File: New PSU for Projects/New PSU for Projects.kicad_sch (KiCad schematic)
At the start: 43 parts, among them IC4 LF351DT, J1 Toroid 5VA/15V, J2 240V Mains, J3 Current Flow Test Point, J4 PVG3A202C01R00, Q1 BC848, Q2 BC848, U3 SN74HC74N

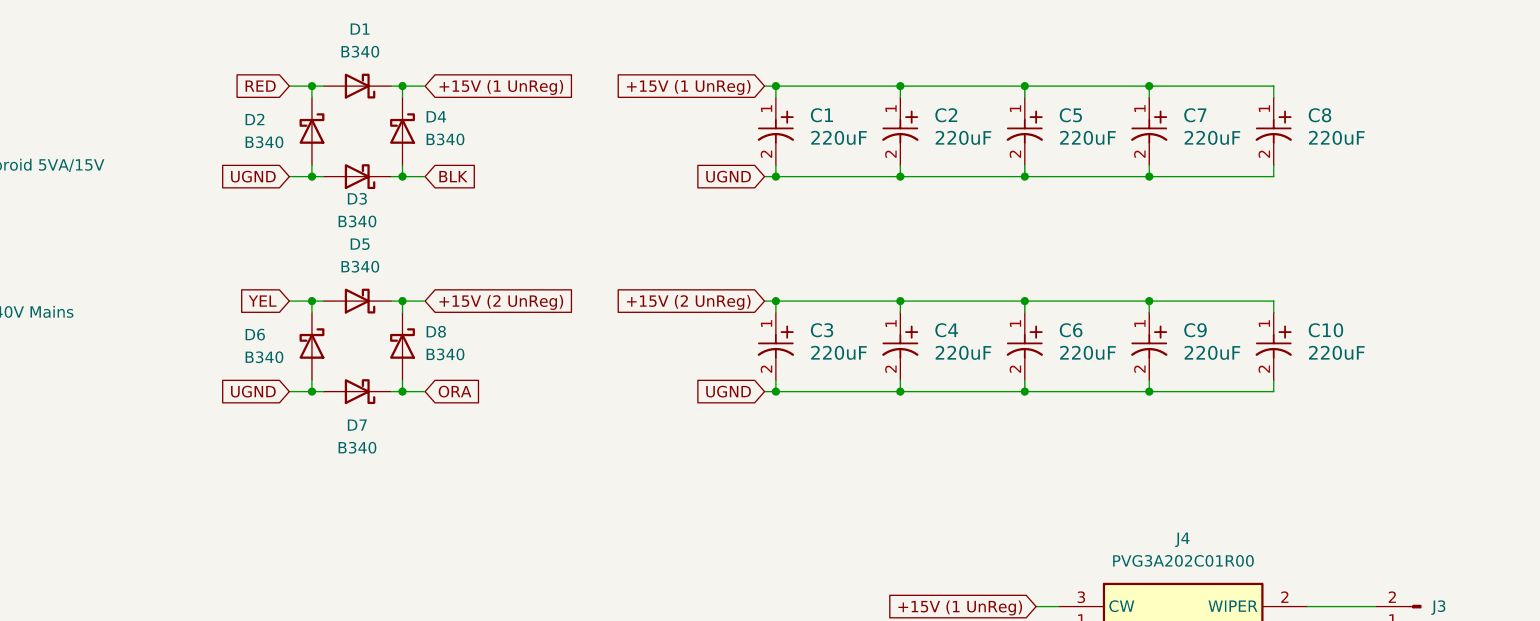
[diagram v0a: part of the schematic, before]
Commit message: A few minor changes
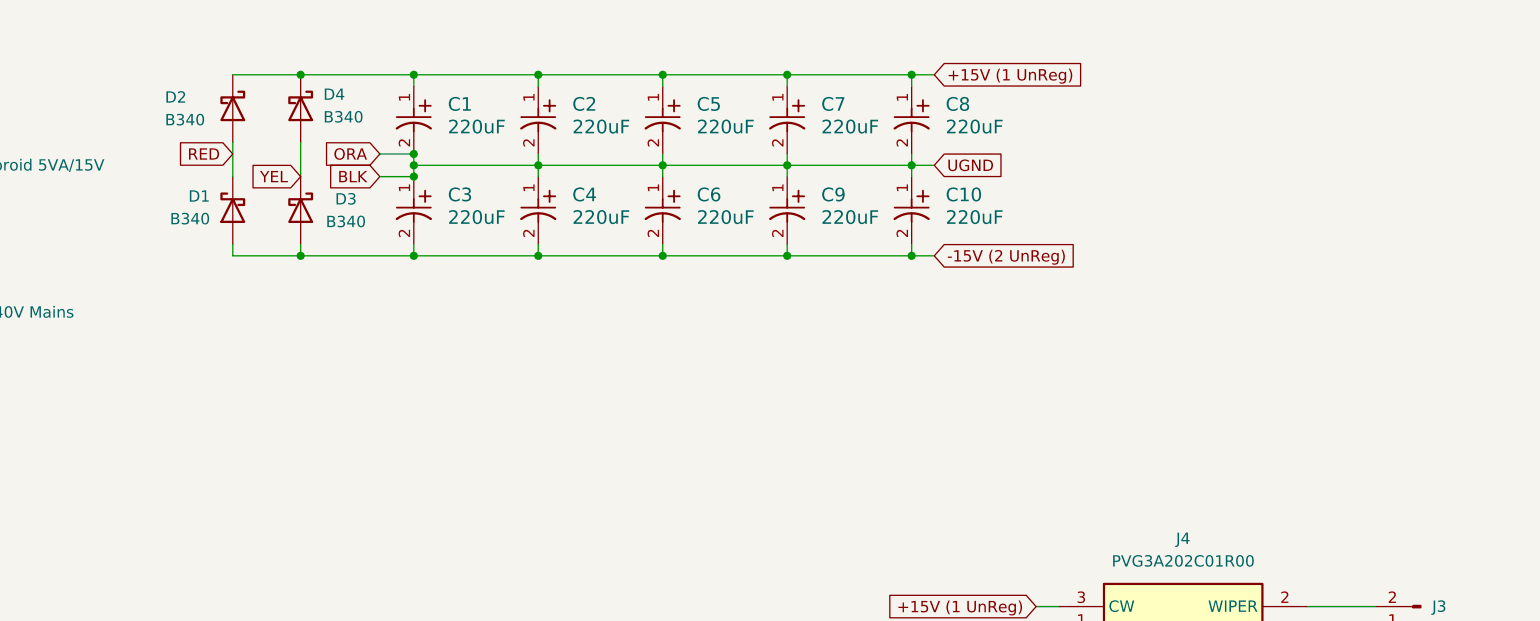
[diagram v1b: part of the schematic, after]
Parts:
- removed D5, D6, D7, D8: B340, Diode_SMD:D_SMC, symbol Diode:B340
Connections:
- net +15V (2 UnReg) is gone; now on net BLK: C10.1, C3.1, C4.1, C6.1, C9.1
- net ORA is gone; now on net BLK: J1.4 (Pin_4)
- net +15V (1 UnReg): now also D2.1 (K); no longer D1.1 (K)
- net BLK: now also C1.2, C13.2, C14.2, C2.2, C3.1, C5.1, C5.2, C7.2, C8.2, IC4.4 (VCC-), Q1.2 (E), Q2.2 (E), R2.1, U3.7 (GND), Z9.2 (A); no longer D3.1 (K), D4.2 (A)
- net RED: now also D1.1 (K), D2.2 (A); no longer D1.2 (A), D2.1 (K)
- net YEL: now also D3.1 (K), D4.2 (A)
- removed net UGND: C1.2, C10.2, C13.2, C14.2, C2.2, C3.1, C3.2, C4.2, C5.1, C5.2, C6.2, C7.2, C8.2, C9.2, D2.2 (A), D3.2 (A), IC4.4 (VCC-), Q1.2 (E), Q2.2 (E), R2.1, U3.7 (GND), Z9.2 (A)
- new net -15V (2 UnReg): C10.2, C3.2, C4.2, C6.2, C9.2, D1.2 (A), D3.2 (A)
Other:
- moved on the sheet: C1, C10, C2, C3, C4, C5, C6, C7, C8, C9, D1, D2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

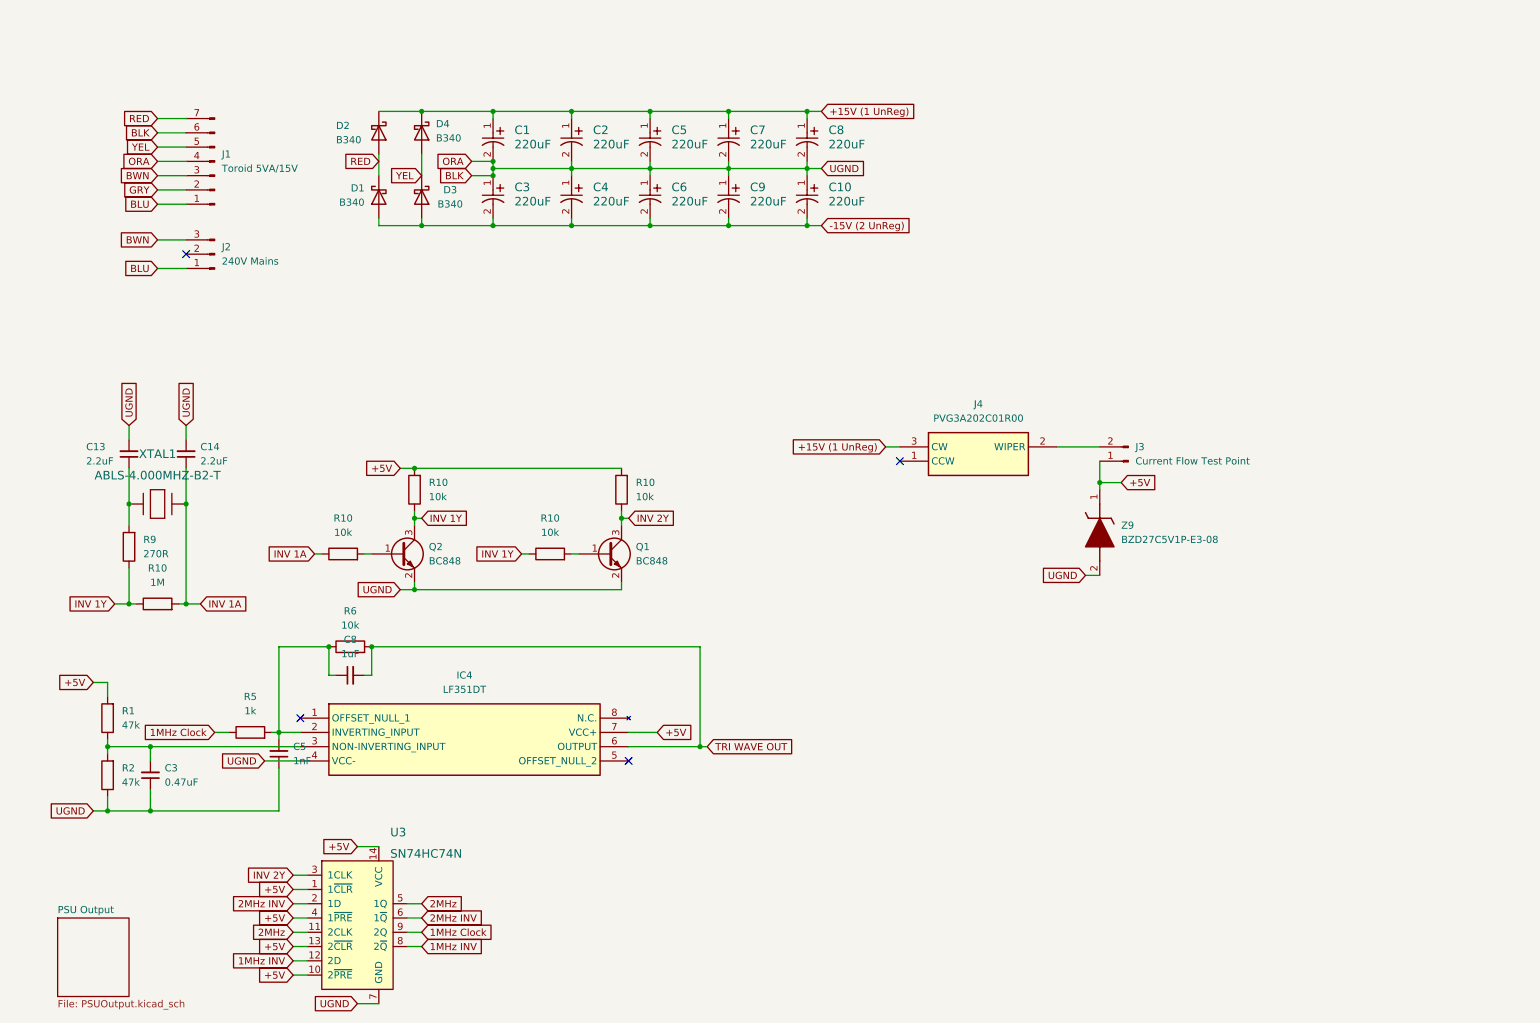
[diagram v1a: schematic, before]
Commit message: Lyrebird Initial Upload
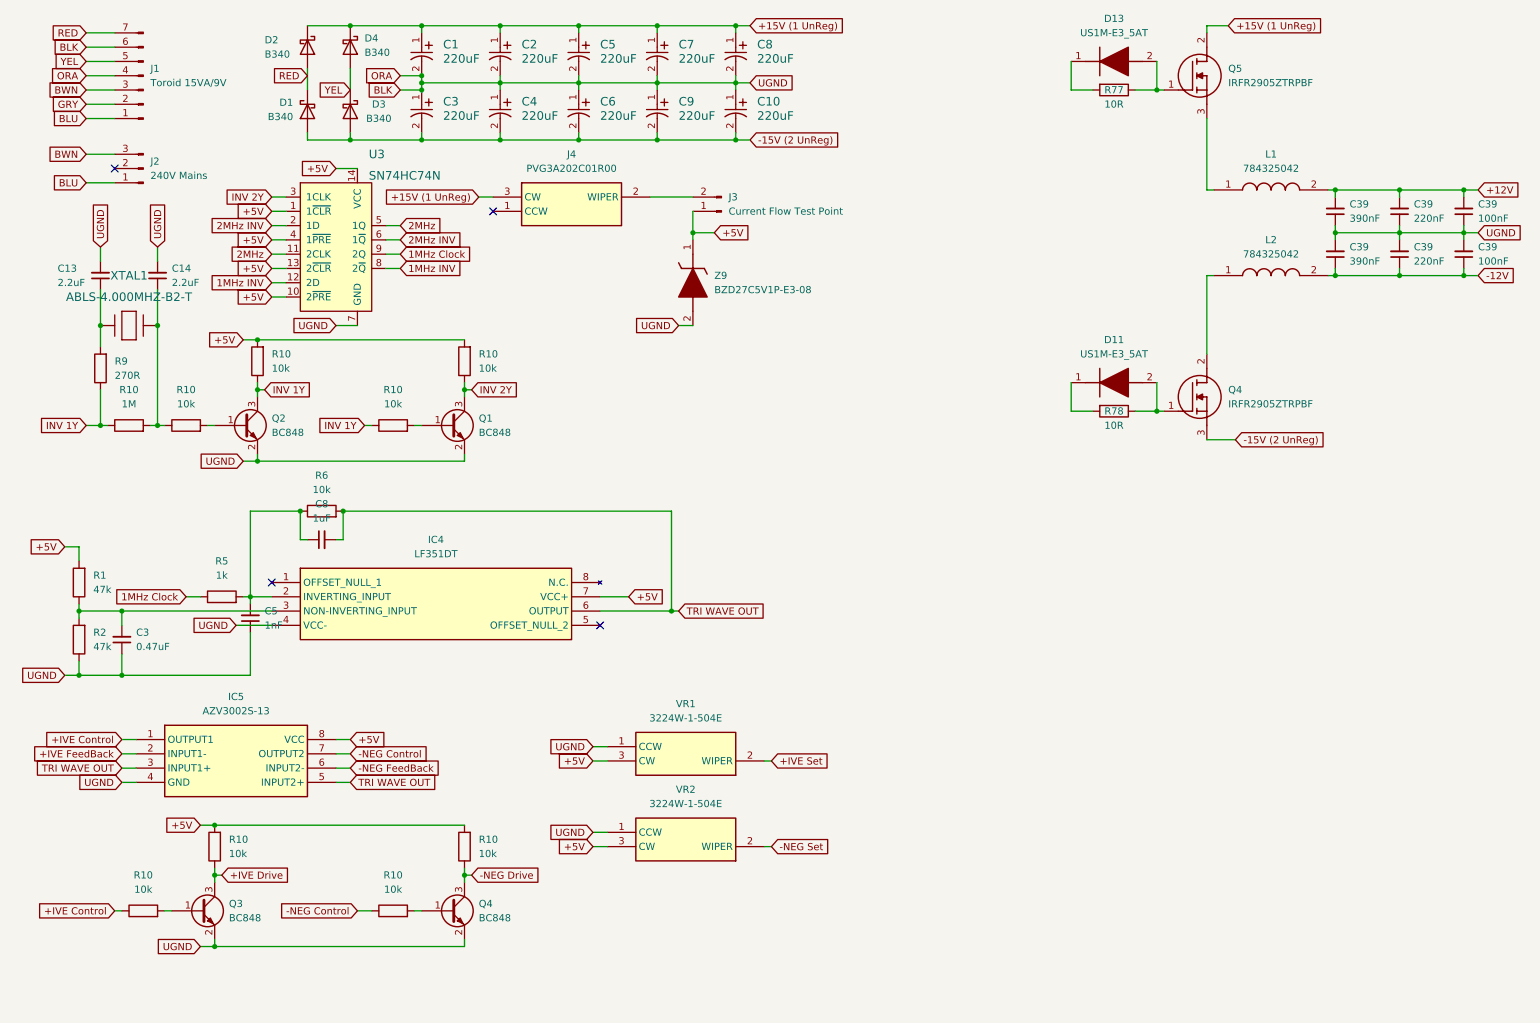
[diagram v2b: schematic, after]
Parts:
- added C39 (x2): 100nF, Capacitor_SMD:C_1206_3216Metric, symbol Device:C_Small
- added C39 (x2): 390nF, Capacitor_SMD:C_1206_3216Metric, symbol Device:C_Small
- added C39 (x2): 220nF, Capacitor_SMD:C_1206_3216Metric, symbol Device:C_Small
- added D11, D13: US1M-E3_5AT, DIOM5127X229N, symbol SamacSys_Parts:US1M-E3_5AT
- added IC5: AZV3002S-13, SOIC127P600X175-8N, symbol SamacSys_Parts:AZV3002S-13
- added L1, L2: 784325042, INDPM105100X463N, symbol SamacSys_Parts:784325042
- added Q3, Q4: BC848, Package_TO_SOT_SMD:SOT-23, symbol Transistor_BJT:BC848
- added Q4, Q5: IRFR2905ZTRPBF, IRFR2905ZTRPBF, symbol SamacSys_Parts:IRFR2905ZTRPBF
- added R10 (x4): 10k, Resistor_SMD:R_1206_3216Metric, symbol Device:R
- added R77, R78: 10R, Resistor_SMD:R_1206_3216Metric, symbol Device:R
- added VR1, VR2: 3224W-1-504E, 3224W1205E, symbol SamacSys_Parts:3224W-1-504E
- J1: value Toroid 5VA/15V -> Toroid 15VA/9V
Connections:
- net +15V (1 UnReg): now also Q5.2 (D)
- net +5V: now also IC5.8 (VCC), R10.2, R10.2, VR1.3 (CW), VR2.3 (CW)
- net -15V (2 UnReg): now also Q4.3 (S)
- net BLK: now also C39.1, C39.1, C39.1, C39.2, C39.2, C39.2, IC5.4 (GND), Q3.2 (E), Q4.2 (E), VR1.1 (CCW), VR2.1 (CCW)
- net TRI WAVE OUT: now also IC5.3 (INPUT1+), IC5.5 (INPUT2+)
- net INV 1A: no longer names the net of C14.1, R10.1, R10.2, XTAL1.2
- new net: Q3.1 (B), R10.2
- new net: D11.2 (A), Q4.1 (G), R78.1
- new net: L2.1, Q4.2 (D)
- new net: D11.1 (K), R78.2
- new net: D13.1 (K), R77.2
- new net: D13.2 (A), Q5.1 (G), R77.1
- new net: L1.1, Q5.3 (S)
- new net: Q4.1 (B), R10.2
- new net +12V: C39.2, C39.2, C39.2, L1.2
- new net +IVE Control: IC5.1 (OUTPUT1), R10.1
- new net +IVE Drive: Q3.3 (C), R10.1
- new net +IVE FeedBack: IC5.2 (INPUT1-)
- new net +IVE Set: VR1.2 (WIPER)
- new net -12V: C39.1, C39.1, C39.1, L2.2
- new net -NEG Control: IC5.7 (OUTPUT2), R10.1
- new net -NEG Drive: Q4.3 (C), R10.1
- new net -NEG FeedBack: IC5.6 (INPUT2-)
- new net -NEG Set: VR2.2 (WIPER)
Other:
- removed sheet PSU Output
- moved on the sheet: C1, C10, C13, C14, C2, C3, C4, C5, C6, C7, C8, C9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
